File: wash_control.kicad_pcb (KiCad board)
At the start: 2 copper layers, 64 parts, among them J1 ValveOUT, J10 PD6, J2 MotorOUT, J3 PumpOUT, J4 220V_IN, J5 ISCP, J6 LedOUT, J7 FloatOUT, J8 SwitchOUT, J9 ButtonOUT, Q1 BT136, Q2 BT136, Q3 BT136, SW1 SW_Push, U1 ATmega8A-AU, U2 MOC3023M, U3 MOC3023M, U4 MOC3023M, Y1 16MHz

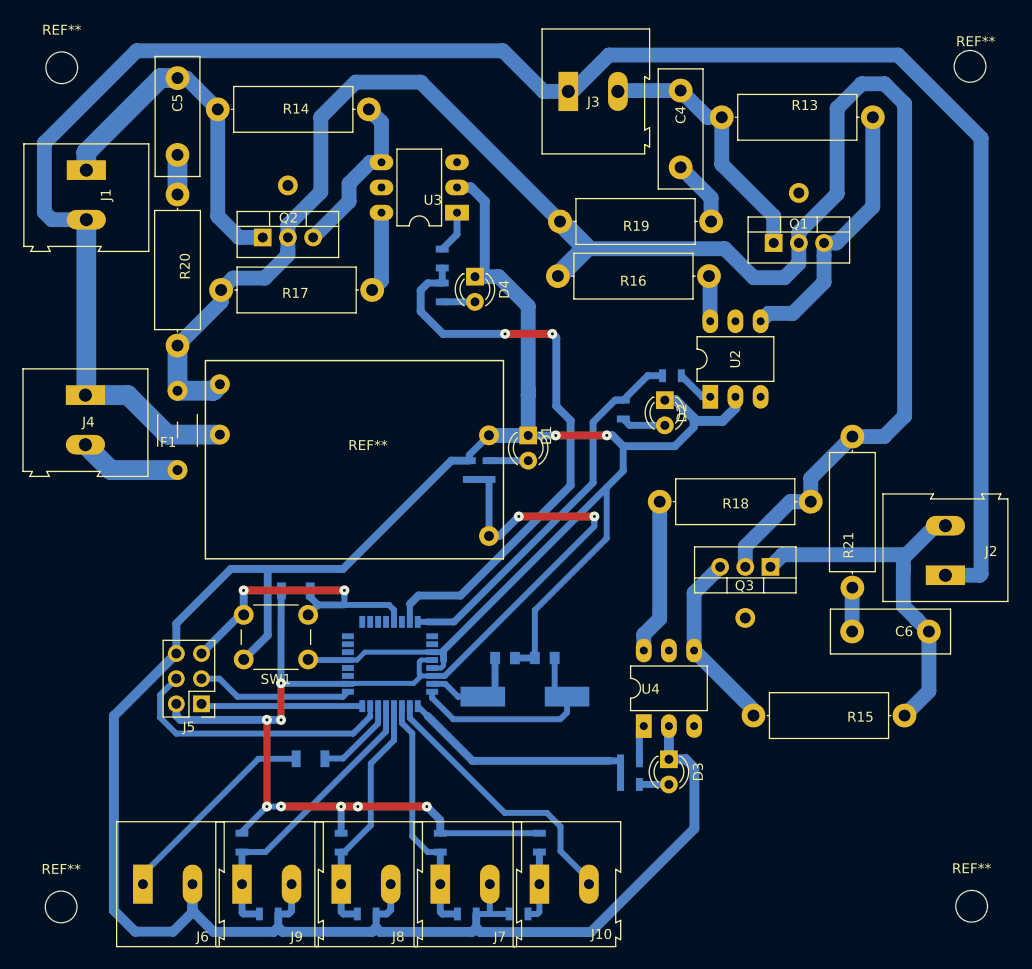
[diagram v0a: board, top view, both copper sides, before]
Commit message: merge
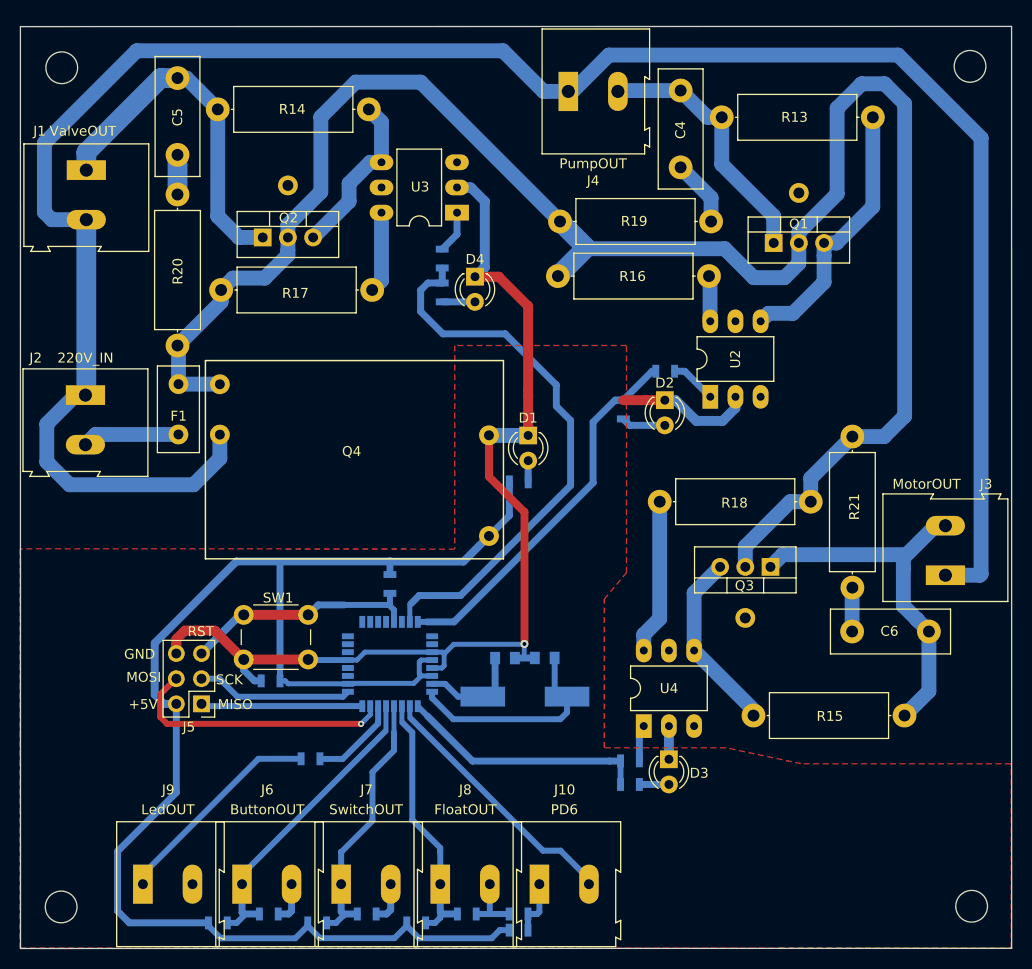
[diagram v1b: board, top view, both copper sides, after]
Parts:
- removed the J2 at (105.3, 67.4)
- added J4: PumpOUT, Connectors_Terminal_Blocks:TerminalBlock_Altech_AK300-2_P5.00mm, F.Cu at (67.3, 18.5)
- F1: footprint Library:MyBladeFuse -> Fuse_Holders_and_Fuses:Fuse_TE5_Littlefuse-395Series
- J3: value PumpOUT -> MotorOUT
- R1, R2: footprint Resistors_SMD:R_1206 -> Resistors_SMD:R_0805
- moved J3 61.9 mm to (105.3, 67.4), turned to 90 degrees
- moved C3 29.2 mm to (37.2, 78.0), turned to 0 degrees
- moved R1 9.52 mm to (49.3, 68.2), turned to 270 degrees
- moved R22 9.08 mm to (62.3, 103.2), turned to 180 degrees
- moved R4 8.46 mm to (31.9, 102.4), turned to 0 degrees
- moved R5 8.46 mm to (51.9, 102.4), turned to 0 degrees
- moved R3 8.45 mm to (42.0, 102.4), turned to 0 degrees
- moved F1 3.59 mm to (27.9, 53.1)
- moved R6 3.23 mm to (62.3, 57.9), turned to 0 degrees
- moved R7 0.82 mm to (77.1, 46.8)
- renumbered J4 to J2, J9 to J6, J8 to J7, J7 to J8, J6 to J9, REF** to Q4
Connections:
- J3 pad 2: /Pump -> /Motor
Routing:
- net Earth: track 315.9 -> 137.5 mm, vias 2 -> 1
- net +5V: track 132.7 -> 151.5 mm, vias 10 -> 0
- net /220_In2: track 197.2 -> 212.8 mm
- net /RST: track 32.2 -> 24.1 mm, vias 2 -> 0
- net /Switch: track 24.9 -> 28.7 mm
- net /ValvePin: track 59.4 -> 56.5 mm, vias 2 -> 0
- net Net-(D1-Pad2): track 3.95 -> 2.14 mm
- net Net-(J10-Pad1): track 7.28 -> 5.67 mm
- net /Float: track 24.9 -> 26.4 mm
- net /PD6: track 27.9 -> 26.4 mm
- net /220_In1: track 184.8 -> 183.8 mm
- net Net-(R7-Pad1): track 3.80 -> 4.67 mm
- net /MOSI: track 28.2 -> 27.4 mm, vias 0 -> 1
- net /Button: track 30.1 -> 30.8 mm
- net Net-(F1-Pad1): track 10.4 -> 9.81 mm
- added copper zone on F.Cu, net Earth
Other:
- board outline added: 100 x 93 mm
- board text added: "+"
- board text added: "+5V"
- board text added: "-"
- board text added: "GND"
- board text added: "MISO"
- board text added: "MOSI"
- board text added: "RST"
- board text added: "SCK"
